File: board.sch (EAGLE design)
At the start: 46 parts, among them IC1 ATMEGA48/88/168-AU, IC2 TP4056, IC3 MAX31865, IC4 MCP1703CB, Q1 PH2925U, Q2 IRLML2244

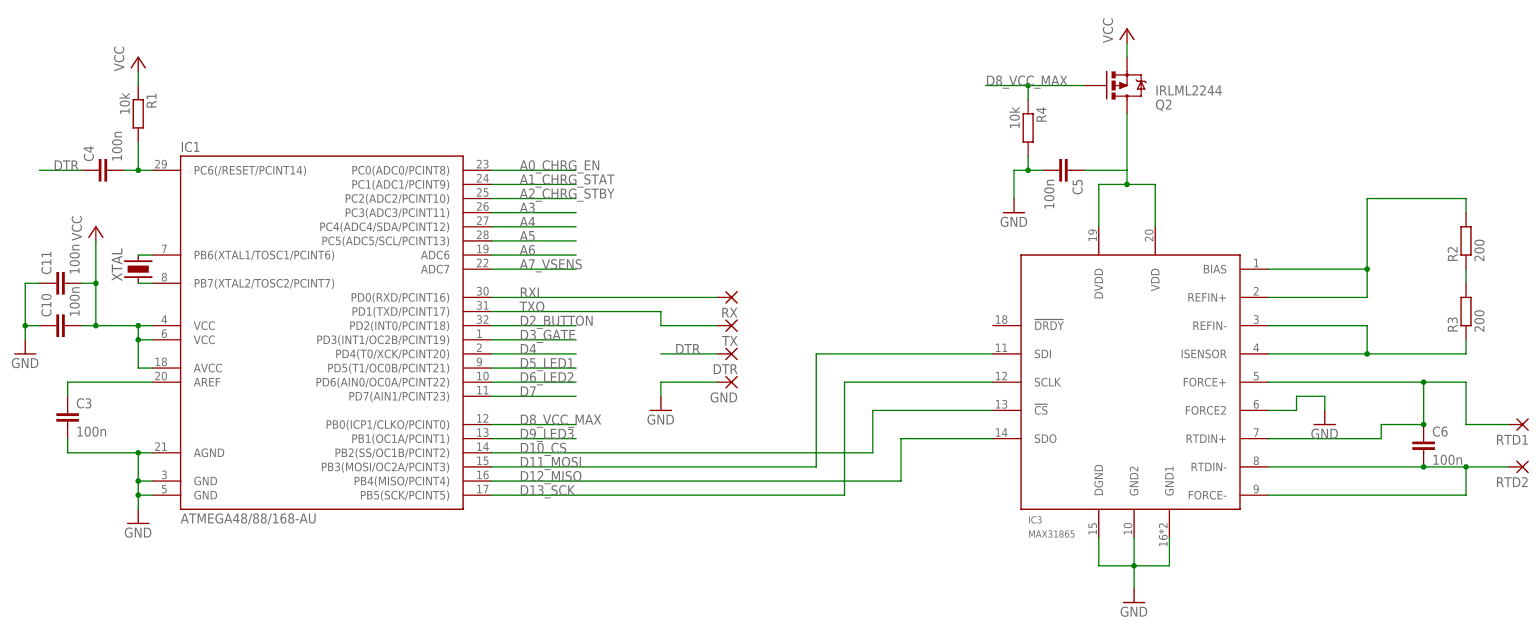
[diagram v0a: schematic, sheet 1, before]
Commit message: draft
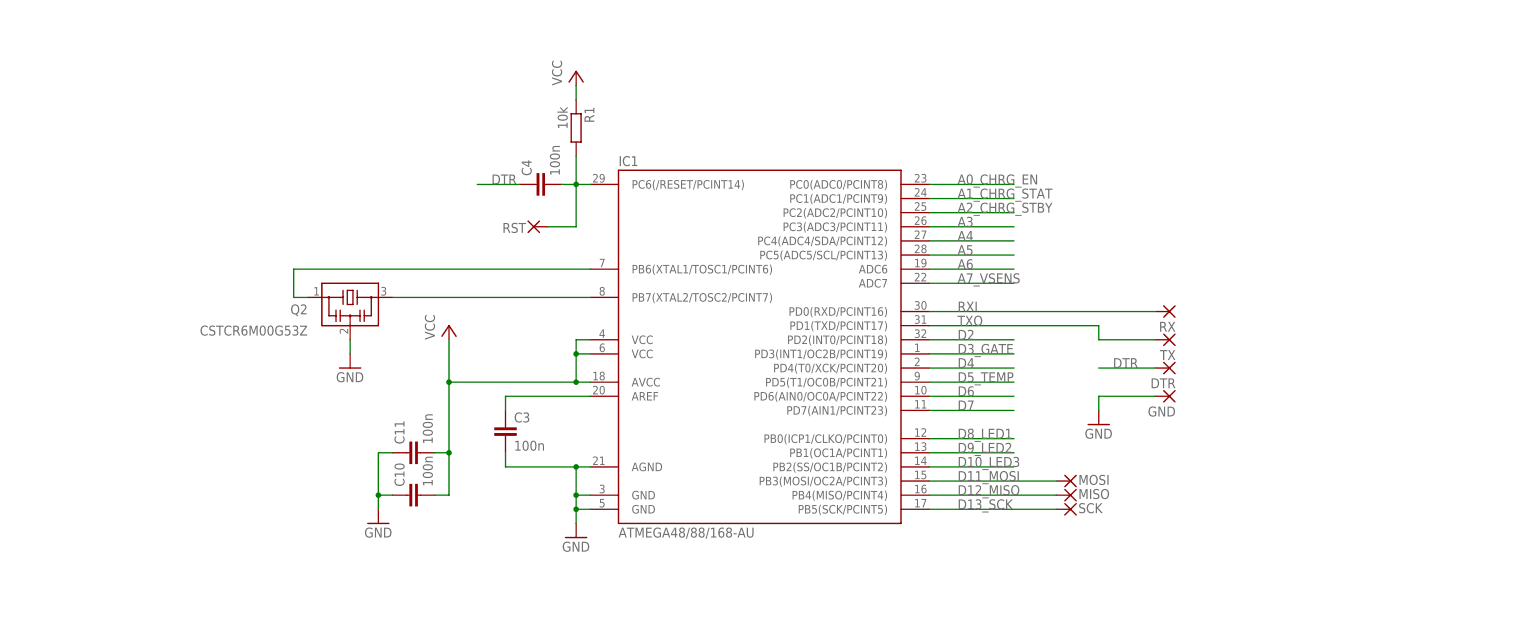
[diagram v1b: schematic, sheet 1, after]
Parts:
- removed C5, C6: 100n, rcl:C-EUC0603
- removed GND_LED: (no value), wirepad:SMD2
- removed IC3: MAX31865, Oles komponentbibliotek:MAX31865
- removed R2, R3: 200, rcl:R-EU_R0603
- removed XTAL: (no value), xtal:XTAL-HCS10
- added MISO, MOSI, RST, SCK, VCC_LED: (no value), wirepad:SMD2
- Q2: value IRLML2244 -> CSTCR6M00G53Z; device SparkFun-DiscreteSemi:MOSFET-PCHANNELIRLML2244 -> murata-filter:CSTCR6M00G53Z
- R4: value 10k -> 500
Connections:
- removed net D10_CS: IC1.PB2(SS/OC1B/PCINT2), IC3.!CS
- removed net D2_BUTTON: BTN1.P, IC1.PD2(INT0/PCINT18)
- removed net D5_LED1: IC1.PD5(T1/OC0B/PCINT21), R5.2
- removed net D6_LED2: IC1.PD6(AIN0/OC0A/PCINT22), R6.2
- removed net D8_VCC_MAX: IC1.PB0(ICP1/CLKO/PCINT0), Q2.G, R4.1
- removed net D9_LED3: IC1.PB1(OC1A/PCINT1), R12.2
- removed net N$5: R2.1, R3.2
- removed net TEMP_IN-: C6.2, IC3.FORCE-, IC3.RTDIN-, RTD2.P
- removed net TEMP_REF+: IC3.BIAS, IC3.REFIN+, R2.2
- removed net TEMP_REF-: IC3.ISENSOR, IC3.REFIN-, R3.1
- removed net VCC_MAX: C5.1, IC3.DVDD, IC3.VDD, Q2.D
- removed net XTAL2: IC1.PB7(XTAL2/TOSC2/PCINT7), XTAL.P1
- new net D10_LED3: IC1.PB2(SS/OC1B/PCINT2), R12.2
- new net D2: IC1.PD2(INT0/PCINT18)
- new net D5_TEMP: IC1.PD5(T1/OC0B/PCINT21)
- new net D6: IC1.PD6(AIN0/OC0A/PCINT22)
- new net D8_LED1: IC1.PB0(ICP1/CLKO/PCINT0), R5.2
- new net D9_LED2: IC1.PB1(OC1A/PCINT1), R6.2
- new net N$1: IC1.PB7(XTAL2/TOSC2/PCINT7), Q2.3
- new net N$2: RTD2.P
- net D11_MOSI: now also MOSI.P; no longer IC3.SDI
- net D12_MISO: now also MISO.P; no longer IC3.SDO
- net D13_SCK: now also SCK.P; no longer IC3.SCLK
- net GND: now also Q2.2; no longer BTN2.P, C5.2, GND_LED.P, IC3.DGND, IC3.FORCE2, IC3.GND1, IC3.GND2, R4.2
- net RST: now also RST.P
- net TEMP_IN+: now also R4.2; no longer C6.1, IC3.FORCE+, IC3.RTDIN+
- net VBAT: now also BTN2.P; no longer BAT+.P
- net VCC: now also BAT+.P, BTN1.P, R4.1, VCC_LED.P; no longer Q2.S
- net XTAL1: now also Q2.1; no longer XTAL.P2
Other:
- note added: "Temperature Sensor"
- note removed: "Button"
- moved on the sheet: BAT+, BAT-, BTN1, BTN2, C10, C11, C3, C4, DTR, GND, IC1, LED1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
